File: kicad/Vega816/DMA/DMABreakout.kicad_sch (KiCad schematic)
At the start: 26 parts, among them J17 VPA/VDA, J18 Conn_02x40_Odd_Even, J19 CPU, J20 8MB, J21 4MB, J22 2MB, J23 1MB, J24 512KB, J25 256KB, J26 128KB, J27 64KB, J28 ~{DMA 1}, J29 ~{DMA 0}, J30 DMA Ctrl, J31 VPA/VDA, J32 Conn_02x40_Odd_Even, J33 DMA, U26 74HC00, U30 74HC08, U31 74HC283

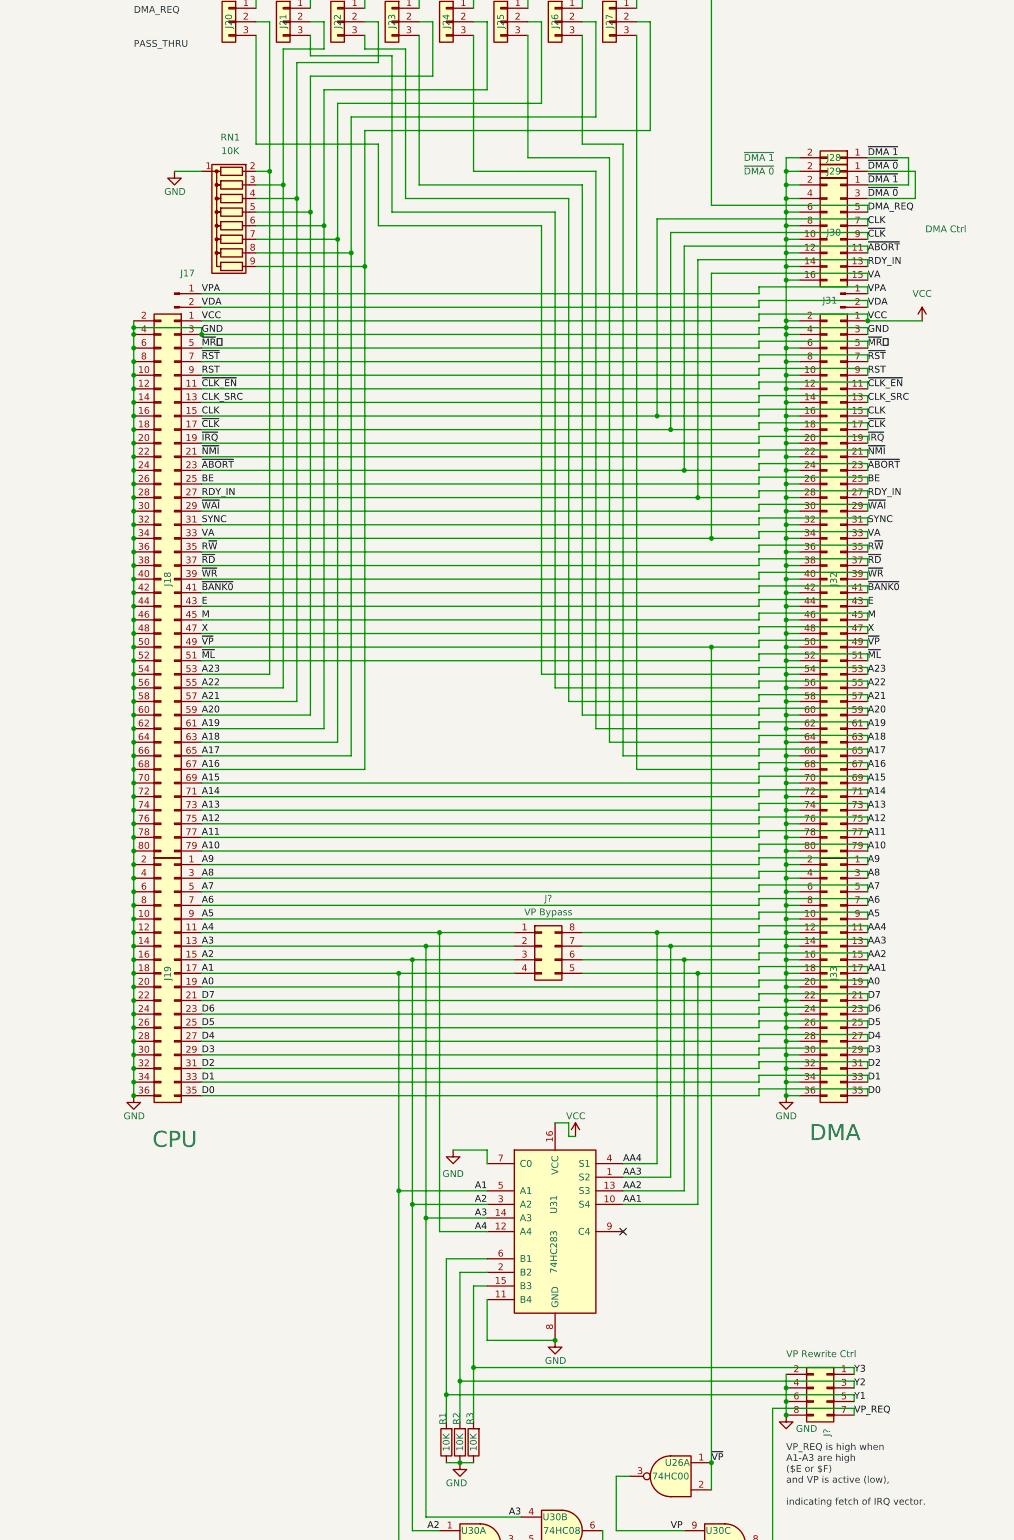
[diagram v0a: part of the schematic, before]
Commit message: irq shim
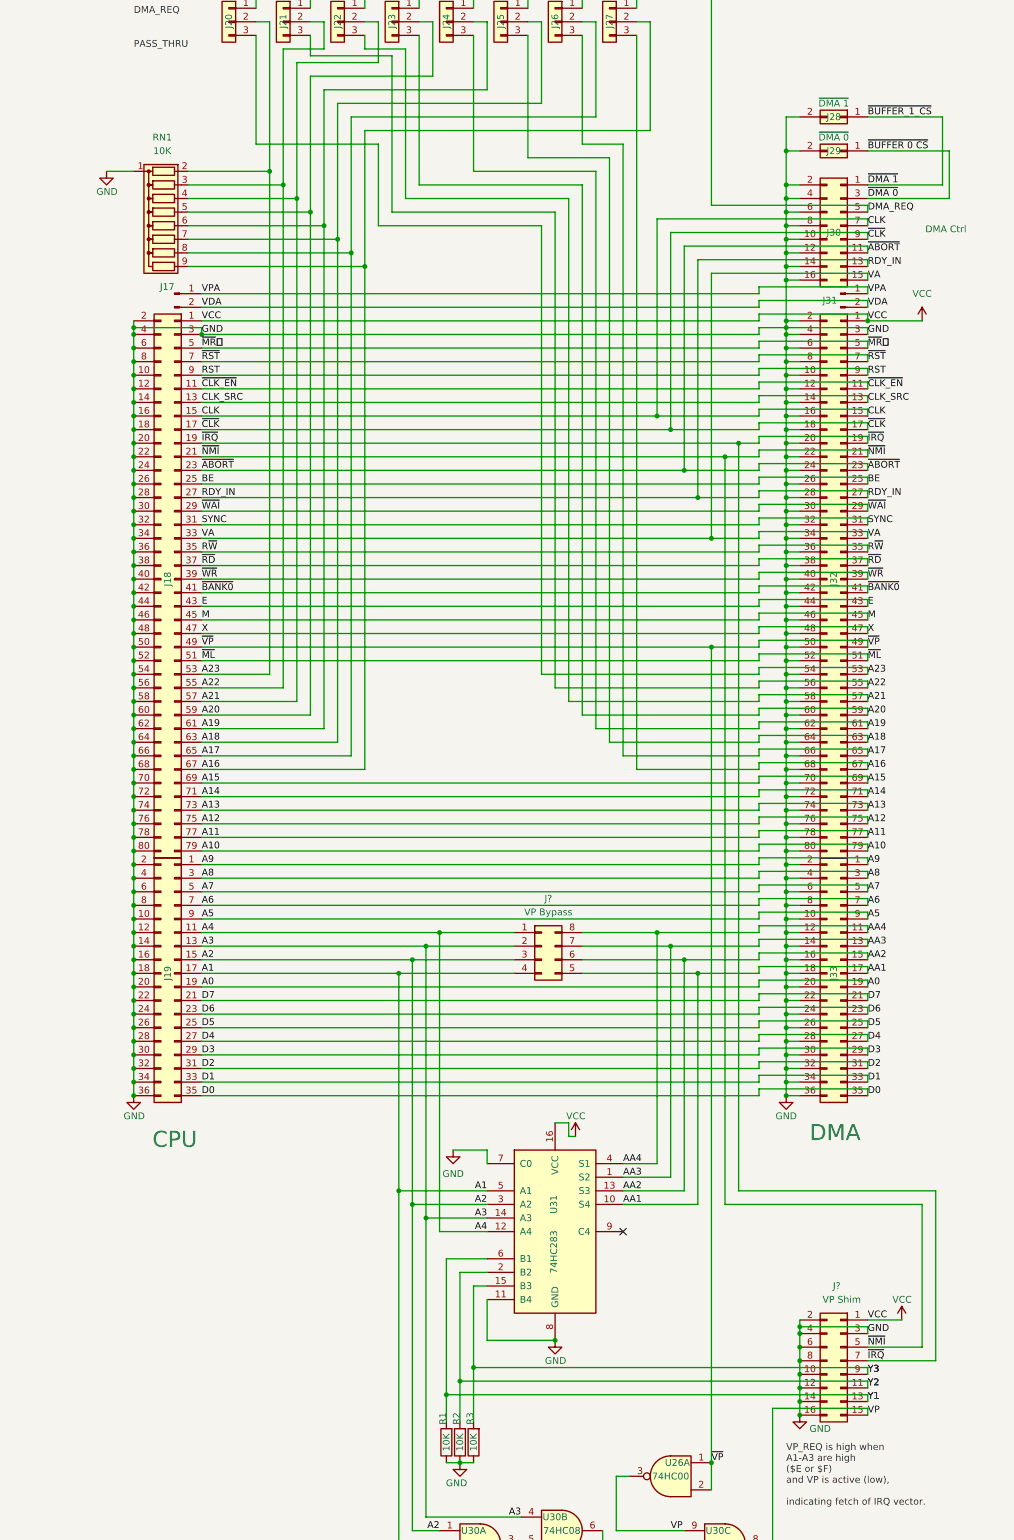
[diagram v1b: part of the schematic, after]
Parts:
- removed J?: VP Rewrite Ctrl, symbol Connector_Generic:Conn_02x04_Odd_Even
- added J?: VP Shim, symbol Connector_Generic:Conn_02x08_Odd_Even
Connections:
- net VP_REQ is gone; now on net VP: U30.8
- net GND: now also J?.10 (Pin_10), J?.12 (Pin_12), J?.14 (Pin_14), J?.16 (Pin_16), J?.2 (Pin_2), J?.3 (Pin_3), J?.4 (Pin_4), J?.6 (Pin_6), J?.8 (Pin_8)
- net VCC: now also J?.1 (Pin_1)
- net VP: now also J?.15 (Pin_15)
- net Y1: now also J?.13 (Pin_13)
- net Y2: now also J?.11 (Pin_11)
- net Y3: now also J?.9 (Pin_9)
- net ~{IRQ}: now also J?.7 (Pin_7)
- net ~{NMI}: now also J?.5 (Pin_5)
- net ~{DMA 0} renamed ~{BUFFER 0 CS}
- net ~{DMA 1} renamed ~{BUFFER_1_CS}
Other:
- moved on the sheet: J28, J29, RN1
